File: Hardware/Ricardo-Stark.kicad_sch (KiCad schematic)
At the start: 53 parts, among them J1 RBUS, J11 Conn_01x08_Socket, J5 Conn_01x03_Socket, U1 ESP32-S3, U14 PCA9534RGVR, Y1 R940000171

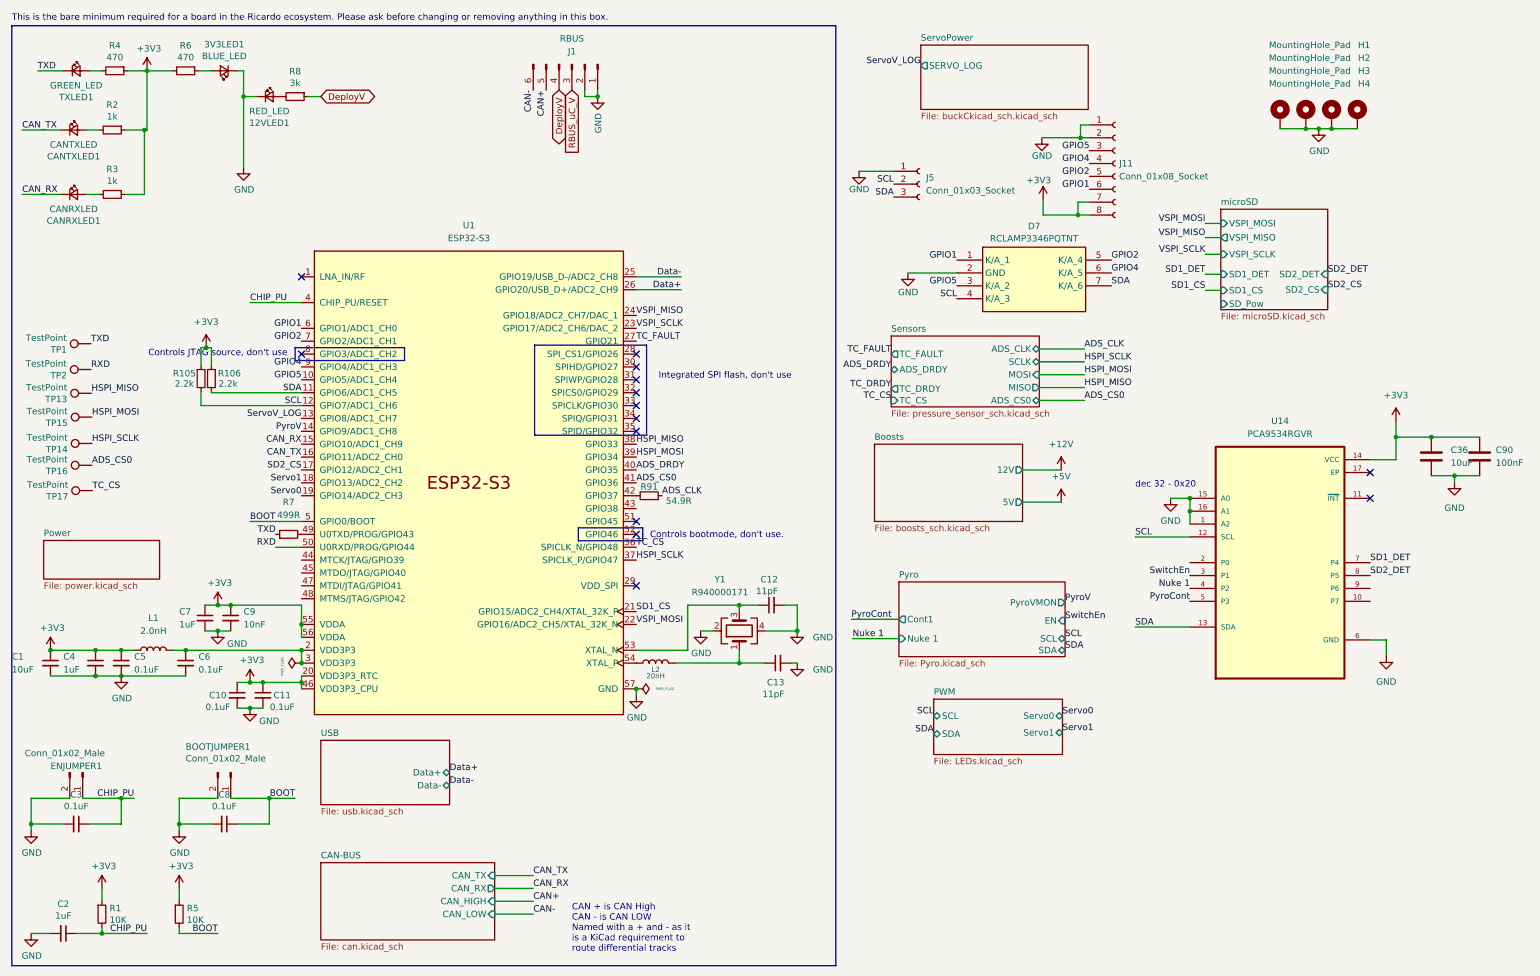
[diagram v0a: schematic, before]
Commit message: v2 Ready for Review
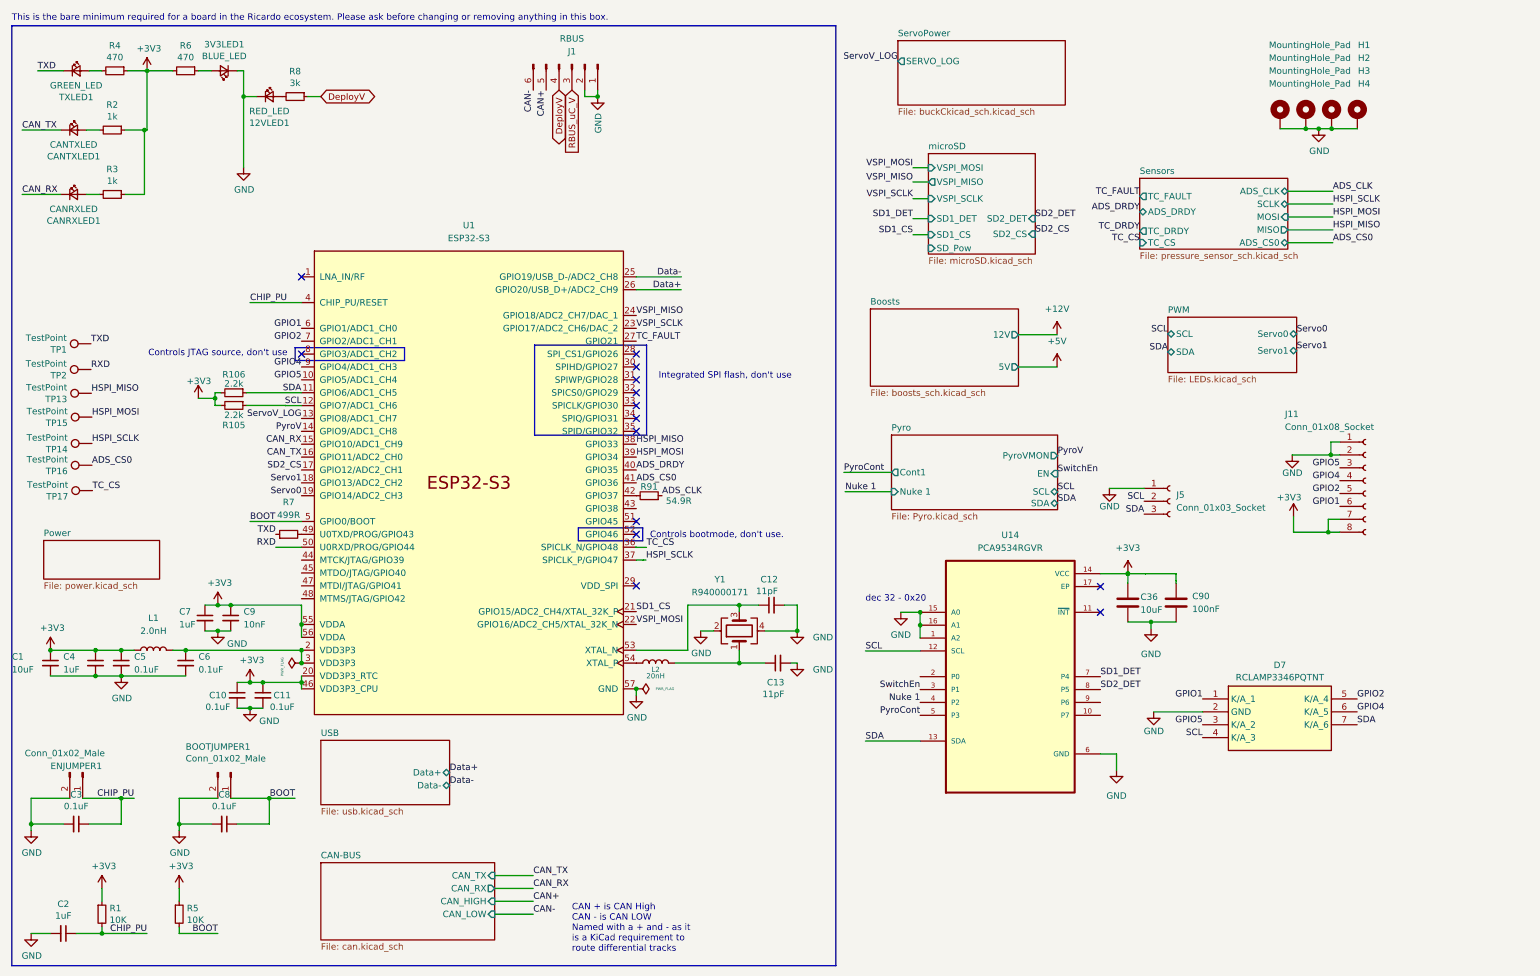
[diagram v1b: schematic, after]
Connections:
- net +3V3: now also R105.2, R106.2; no longer R105.1, R106.1
- net SCL: now also R105.1; no longer R105.2
- net SDA: now also R106.1; no longer R106.2, U1.11 (GPIO6/ADC1_CH5)
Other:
- moved on the sheet: C36, C90, D7, J11, J5, R105, R106, U14
